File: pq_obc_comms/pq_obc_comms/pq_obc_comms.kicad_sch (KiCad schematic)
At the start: 70 parts, among them J1 Conn_01x10, J2 Conn_01x10, J3 Conn_01x10, J4 Conn_01x10, J6 U.FL, U1 STM32L476RGTx, U2 SX1262IMLTRT, U3 BD2232G-GTR, U4 BD2232G-GTR, U5 BGS12PL6E6327XTSA1, U6 BD2232G-GTR, U7 BD2232G-GTR, X1 ECS-120-18-33-JEM-TR3, X2 FA-128_32.0000MF20X-K5, X3 ABS09-32.768KHZ-7-T

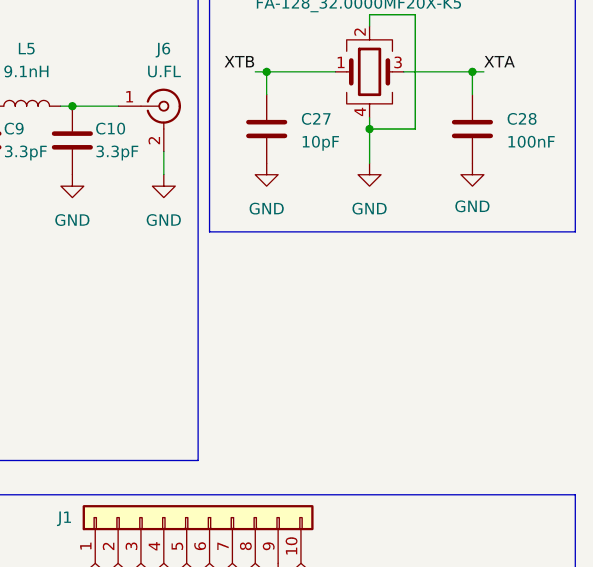
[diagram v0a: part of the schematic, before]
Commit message: Functional revision and finishing touches part II
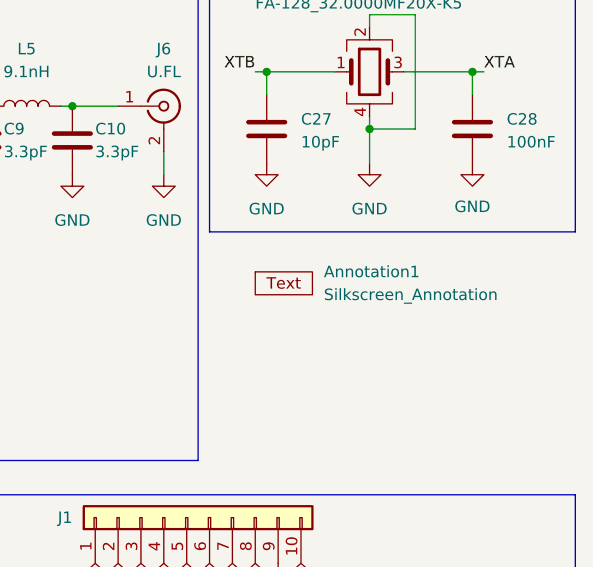
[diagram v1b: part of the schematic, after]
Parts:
- added Annotation1: Silkscreen_Annotation, symbols-nsl:Bike, symbol symbols-nsl:Silkscreen_Annotation
- U5: footprint GGS_RF:PG-TSLP-6-4 -> rf-nsl:PG-TSLP-6-4
- X1: footprint GGS_Miscellaneous:ECX-32 -> miscelaneous-nsl:ECX-32
- X2: footprint GGS_Miscellaneous:EPSON_FA128 -> miscelaneous-nsl:EPSON_FA128
- X3: footprint GGS_Miscellaneous:ABS09 -> miscelaneous-nsl:ABS09
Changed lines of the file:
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@@
     (pin "1")
   )
+  (symbol (lib_id "symbols-nsl:Silkscreen_Annotation") (at 247.65 58.42 0) (unit 1)
+    (in_bom yes) (on_board yes) (fields_autoplaced)
+    (property "Reference" "Annotation1" (id 0) (at 254 51.4349 0)
+      (effects (font (size 1.27 1.27)) (justify left))
+    )
+    (property "Value" "Silkscreen_Annotation" (id 1) (at 254 53.9749 0)
+      (effects (font (size 1.27 1.27)) (justify left))
+    )
+    (property "Footprint" "symbols-nsl:Bike" (id 2) (at 247.65 58.42 0)
+      (effects (font (size 1.27 1.27)) hide)
+    )
+    (property "Datasheet" "" (id 3) (at 247.65 58.42 0)
+      (effects (font (size 1.27 1.27)) hide)
+    )
+  )
   (symbol (lib_id "power:GND") (at 116.84 25.4 0) (unit 1)
     (in_bom yes) (on_board yes)
@@
     (property "Reference" "U5" (id 0) (at 184.15 22.86 0))
     (property "Value" "BGS12PL6E6327XTSA1" (id 1) (at 184.15 25.4 0))
-    (property "Footprint" "GGS_RF:PG-TSLP-6-4" (id 2) (at 184.15 33.02 0)
+    (property "Footprint" "rf-nsl:PG-TSLP-6-4" (id 2) (at 184.15 33.02 0)
       (effects (font (size 1.27 1.27)) hide)
     )
@@
       (effects (font (size 1.27 1.27)) (justify left))
     )
-    (property "Footprint" "GGS_Miscellaneous:EPSON_FA128" (id 2) (at 259.08 29.21 0)
+    (property "Footprint" "miscelaneous-nsl:EPSON_FA128" (id 2) (at 259.08 29.21 0)
       (effects (font (size 1.27 1.27)) hide)
     )
@@
     (property "Reference" "X3" (id 0) (at 219.71 142.24 0))
     (property "Value" "ABS09-32.768KHZ-7-T" (id 1) (at 219.71 144.78 0))
-    (property "Footprint" "GGS_Miscellaneous:ABS09" (id 2) (at 219.71 148.59 0)
+    (property "Footprint" "miscelaneous-nsl:ABS09" (id 2) (at 219.71 148.59 0)
       (effects (font (size 1.27 1.27)) hide)
     )
@@
       (effects (font (size 1.27 1.27)) (justify left))
     )
-    (property "Footprint" "GGS_Miscellaneous:ECX-32" (id 2) (at 260.35 151.13 0)
+    (property "Footprint" "miscelaneous-nsl:ECX-32" (id 2) (at 260.35 151.13 0)
       (effects (font (size 1.27 1.27)) hide)
     )
@@
       (reference "#PWR0149") (unit 1) (value "GND") (footprint "")
     )
+    (path "/0e0a9cdf-3063-4090-b911-679c5a730d38"
+      (reference "Annotation1") (unit 1) (value "Silkscreen_Annotation") (footprint "symbols-nsl:Bike")
+    )
     (path "/70f6326e-6380-4875-aac5-5e40eda2ece8"
       (reference "C1") (unit 1) (value "47nF") (footprint "Capacitor_SMD:C_0402_1005Metric")
@@
     )
     (path "/1e73ef1c-3a42-4d69-9bb9-affa28519ebc"
-      (reference "U5") (unit 1) (value "BGS12PL6E6327XTSA1") (footprint "GGS_RF:PG-TSLP-6-4")
+      (reference "U5") (unit 1) (value "BGS12PL6E6327XTSA1") (footprint "rf-nsl:PG-TSLP-6-4")
     )
     (path "/5b2c5bc3-5fa8-4d93-ab7a-d6c8c3adc44e"
@@
     )
     (path "/aee54727-eead-440f-9fa9-5ccf5d66a20e"
-      (reference "X1") (unit 1) (value "ECS-120-18-33-JEM-TR3") (footprint "GGS_Miscellaneous:ECX-32")
+      (reference "X1") (unit 1) (value "ECS-120-18-33-JEM-TR3") (footprint "miscelaneous-nsl:ECX-32")
     )
     (path "/7ef30fbc-71e7-4186-a1d8-48087b5069c5"
-      (reference "X2") (unit 1) (value "FA-128_32.0000MF20X-K5") (footprint "GGS_Miscellaneous:EPSON_FA128")
+      (reference "X2") (unit 1) (value "FA-128_32.0000MF20X-K5") (footprint "miscelaneous-nsl:EPSON_FA128")
     )
     (path "/89691019-6129-4efd-9407-b4187a9c6ccc"
-      (reference "X3") (unit 1) (value "ABS09-32.768KHZ-7-T") (footprint "GGS_Miscellaneous:ABS09")
+      (reference "X3") (unit 1) (value "ABS09-32.768KHZ-7-T") (footprint "miscelaneous-nsl:ABS09")
     )
   )
